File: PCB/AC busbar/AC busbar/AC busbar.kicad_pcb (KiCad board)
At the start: 2 copper layers, 110 x 50 mm, 4 parts

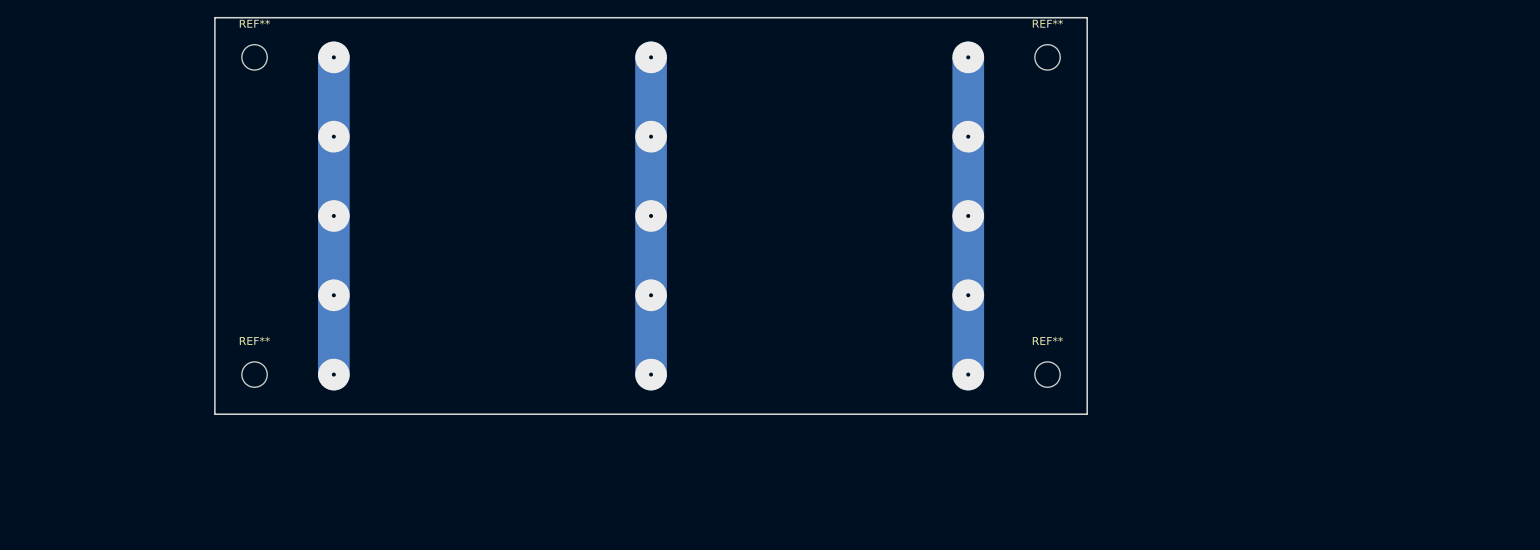
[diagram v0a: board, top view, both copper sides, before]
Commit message: Big commit after a long time :)
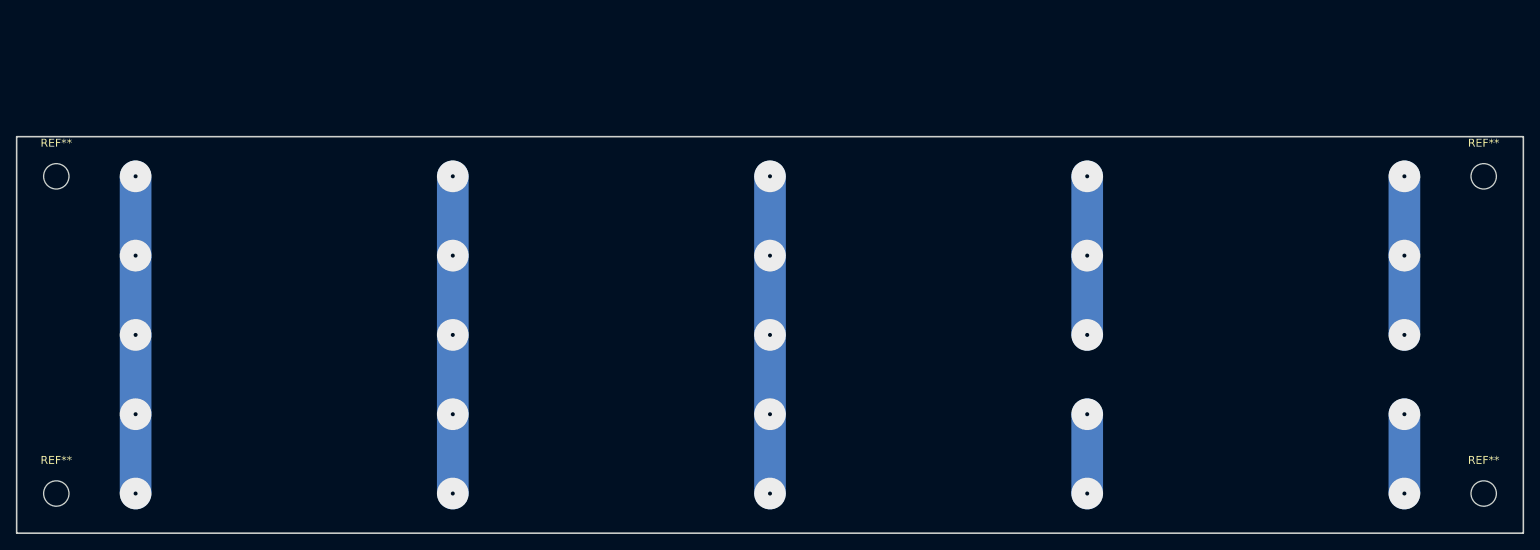
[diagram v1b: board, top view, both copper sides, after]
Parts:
- moved REF** 57.0 mm to (245.0, 65.0)
- moved REF** 57.0 mm to (245.0, 105.0)
- moved REF** 29.2 mm to (65.0, 105.0)
- moved REF** 29.2 mm to (65.0, 65.0)
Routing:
- net (no net): track 0.00 -> 180.0 mm, vias 0 -> 25
- net PE: track 40.0 -> 0.00 mm, vias 5 -> 0
- net N: track 40.0 -> 0.00 mm, vias 5 -> 0
- net L: track 40.0 -> 0.00 mm, vias 5 -> 0
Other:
- board size 110 x 50 mm -> 190 x 50 mm
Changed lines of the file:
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@@
 	)
 	(paper "A4")
+	(title_block
+		(title "Terminals")
+	)
 	(layers
 		(0 "F.Cu" signal)
@@
 	)
 	(net 0 "")
-	(net 1 "L")
-	(net 2 "N")
-	(net 3 "PE")
 	(footprint "MountingHole:MountingHole_3.2mm_M3"
 		(layer "F.Cu")
-		(at 190 50)
+		(at 245 65)
 		(descr "Mounting Hole 3.2mm, no annular, M3")
 		(tags "mounting hole 3.2mm no annular m3")
@@
 	(footprint "MountingHole:MountingHole_3.2mm_M3"
 		(layer "F.Cu")
-		(at 190 90)
+		(at 245 105)
 		(descr "Mounting Hole 3.2mm, no annular, M3")
 		(tags "mounting hole 3.2mm no annular m3")
@@
 	(footprint "MountingHole:MountingHole_3.2mm_M3"
 		(layer "F.Cu")
-		(at 90 90)
+		(at 65 105)
 		(descr "Mounting Hole 3.2mm, no annular, M3")
 		(tags "mounting hole 3.2mm no annular m3")
@@
 	(footprint "MountingHole:MountingHole_3.2mm_M3"
 		(layer "F.Cu")
-		(at 90 50)
+		(at 65 65)
 		(descr "Mounting Hole 3.2mm, no annular, M3")
 		(tags "mounting hole 3.2mm no annular m3")
@@
 	)
 	(gr_rect
-		(start 85 45)
-		(end 195 95)
+		(start 60 60)
+		(end 250 110)
 		(stroke
 			(width 0.2)
@@
 	)
 	(via
-		(at 100 50)
-		(size 4)
-		(drill 0.5)
-		(layers "F.Cu" "B.Cu")
-		(net 1)
-	)
-	(via
-		(at 100 80)
-		(size 4)
-		(drill 0.5)
-		(layers "F.Cu" "B.Cu")
-		(net 1)
-	)
-	(via
-		(at 100 70)
-		(size 4)
-		(drill 0.5)
-		(layers "F.Cu" "B.Cu")
-		(net 1)
-	)
-	(via
-		(at 100 60)
-		(size 4)
-		(drill 0.5)
-		(layers "F.Cu" "B.Cu")
-		(net 1)
-	)
-	(via
-		(at 100 90)
-		(size 4)
-		(drill 0.5)
-		(layers "F.Cu" "B.Cu")
-		(net 1)
+		(at 115 105)
+		(size 4)
+		(drill 0.5)
+		(layers "F.Cu" "B.Cu")
+		(net 0)
+	)
+	(via
+		(at 155 95)
+		(size 4)
+		(drill 0.5)
+		(layers "F.Cu" "B.Cu")
+		(net 0)
+	)
+	(via
+		(at 235 95)
+		(size 4)
+		(drill 0.5)
+		(layers "F.Cu" "B.Cu")
+		(net 0)
+	)
+	(via
+		(at 75 65)
+		(size 4)
+		(drill 0.5)
+		(layers "F.Cu" "B.Cu")
+		(net 0)
+	)
+	(via
+		(at 155 85)
+		(size 4)
+		(drill 0.5)
+		(layers "F.Cu" "B.Cu")
+		(net 0)
+	)
+	(via
+		(at 75 95)
+		(size 4)
+		(drill 0.5)
+		(layers "F.Cu" "B.Cu")
+		(net 0)
+	)
+	(via
+		(at 235 85)
+		(size 4)
+		(drill 0.5)
+		(layers "F.Cu" "B.Cu")
+		(net 0)
+	)
+	(via
+		(at 115 65)
+		(size 4)
+		(drill 0.5)
+		(layers "F.Cu" "B.Cu")
+		(net 0)
+	)
+	(via
+		(at 155 65)
+		(size 4)
+		(drill 0.5)
+		(layers "F.Cu" "B.Cu")
+		(net 0)
+	)
+	(via
+		(at 115 85)
+		(size 4)
+		(drill 0.5)
+		(layers "F.Cu" "B.Cu")
+		(net 0)
+	)
+	(via
+		(at 195 95)
+		(size 4)
+		(drill 0.5)
+		(layers "F.Cu" "B.Cu")
+		(net 0)
+	)
+	(via
+		(at 195 75)
+		(size 4)
+		(drill 0.5)
+		(layers "F.Cu" "B.Cu")
+		(net 0)
+	)
+	(via
+		(at 235 105)
+		(size 4)
+		(drill 0.5)
+		(layers "F.Cu" "B.Cu")
+		(net 0)
+	)
+	(via
+		(at 115 75)
+		(size 4)
+		(drill 0.5)
+		(layers "F.Cu" "B.Cu")
+		(net 0)
+	)
+	(via
+		(at 155 105)
+		(size 4)
+		(drill 0.5)
+		(layers "F.Cu" "B.Cu")
+		(net 0)
+	)
+	(via
+		(at 235 65)
+		(size 4)
+		(drill 0.5)
+		(layers "F.Cu" "B.Cu")
+		(net 0)
+	)
+	(via
+		(at 75 85)
+		(size 4)
+		(drill 0.5)
+		(layers "F.Cu" "B.Cu")
+		(net 0)
+	)
+	(via
+		(at 155 75)
+		(size 4)
+		(drill 0.5)
+		(layers "F.Cu" "B.Cu")
+		(net 0)
+	)
+	(via
+		(at 115 95)
+		(size 4)
+		(drill 0.5)
+		(layers "F.Cu" "B.Cu")
+		(net 0)
+	)
+	(via
+		(at 75 75)
+		(size 4)
+		(drill 0.5)
+		(layers "F.Cu" "B.Cu")
+		(net 0)
+	)
+	(via
+		(at 235 75)
+		(size 4)
+		(drill 0.5)
+		(layers "F.Cu" "B.Cu")
+		(net 0)
+	)
+	(via
+		(at 195 65)
+		(size 4)
+		(drill 0.5)
+		(layers "F.Cu" "B.Cu")
+		(net 0)
+	)
+	(via
+		(at 195 105)
+		(size 4)
+		(drill 0.5)
+		(layers "F.Cu" "B.Cu")
+		(net 0)
+	)
+	(via
+		(at 75 105)
+		(size 4)
+		(drill 0.5)
+		(layers "F.Cu" "B.Cu")
+		(net 0)
+	)
+	(via
+		(at 195 85)
+		(size 4)
+		(drill 0.5)
+		(layers "F.Cu" "B.Cu")
+		(net 0)
 	)
 	(segment
-		(start 100 50)
-		(end 100 90)
+		(start 195 65)
+		(end 195 85)
 		(width 4)
 		(layer "B.Cu")
-		(net 1)
-	)
-	(via
-		(at 180 80)
-		(size 4)
-		(drill 0.5)
-		(layers "F.Cu" "B.Cu")
-		(net 2)
-	)
-	(via
-		(at 180 70)
-		(size 4)
-		(drill 0.5)
-		(layers "F.Cu" "B.Cu")
-		(net 2)
-	)
-	(via
-		(at 180 50)
-		(size 4)
-		(drill 0.5)
-		(layers "F.Cu" "B.Cu")
-		(net 2)
-	)
-	(via
-		(at 180 90)
-		(size 4)
-		(drill 0.5)
-		(layers "F.Cu" "B.Cu")
-		(net 2)
-	)
-	(via
-		(at 180 60)
-		(size 4)
-		(drill 0.5)
-		(layers "F.Cu" "B.Cu")
-		(net 2)
+		(net 0)
 	)
 	(segment
-		(start 180 50)
-		(end 180 90)
+		(start 155 85)
+		(end 155 105)
 		(width 4)
 		(layer "B.Cu")
-		(net 2)
-	)
-	(via
-		(at 140 90)
-		(size 4)
-		(drill 0.5)
-		(layers "F.Cu" "B.Cu")
-		(net 3)
-	)
-	(via
-		(at 140 50)
-		(size 4)
-		(drill 0.5)
-		(layers "F.Cu" "B.Cu")
-		(net 3)
-	)
-	(via
-		(at 140 70)
-		(size 4)
-		(drill 0.5)
-		(layers "F.Cu" "B.Cu")
-		(net 3)
-	)
-	(via
-		(at 140 60)
-		(size 4)
-		(drill 0.5)
-		(layers "F.Cu" "B.Cu")
-		(net 3)
-	)
-	(via
-		(at 140 80)
-		(size 4)
-		(drill 0.5)
-		(layers "F.Cu" "B.Cu")
-		(net 3)
+		(net 0)
 	)
 	(segment
-		(start 140 50)
-		(end 140 90)
+		(start 235 95)
+		(end 235 105)
 		(width 4)
 		(layer "B.Cu")
-		(net 3)
+		(net 0)
+	)
+	(segment
+		(start 235 65)
+		(end 235 85)
+		(width 4)
+		(layer "B.Cu")
+		(net 0)
+	)
+	(segment
+		(start 115 65)
+		(end 115 105)
+		(width 4)
+		(layer "B.Cu")
+		(net 0)
+	)
+	(segment
+		(start 155 65)
+		(end 155 85)
+		(width 4)
+		(layer "B.Cu")
+		(net 0)
+	)
+	(segment
+		(start 75 65)
+		(end 75 105)
+		(width 4)
+		(layer "B.Cu")
+		(net 0)
+	)
+	(segment
+		(start 195 95)
+		(end 195 105)
+		(width 4)
+		(layer "B.Cu")
+		(net 0)
 	)
 )
